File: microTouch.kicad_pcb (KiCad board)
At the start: 2 copper layers, 26.7 x 41.9 mm, 9 parts, among them J1 SERVO, J2 PRINTER, U1 T1302

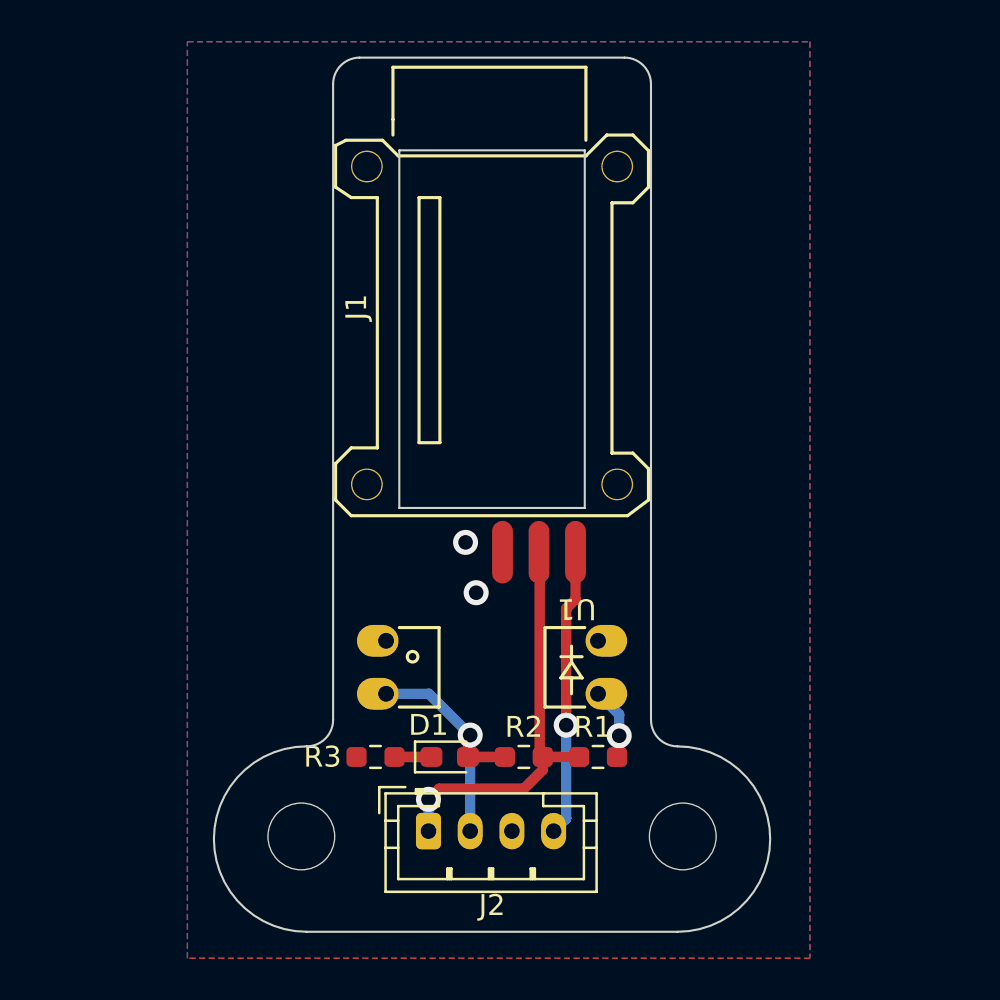
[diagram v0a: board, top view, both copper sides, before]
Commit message: smaller
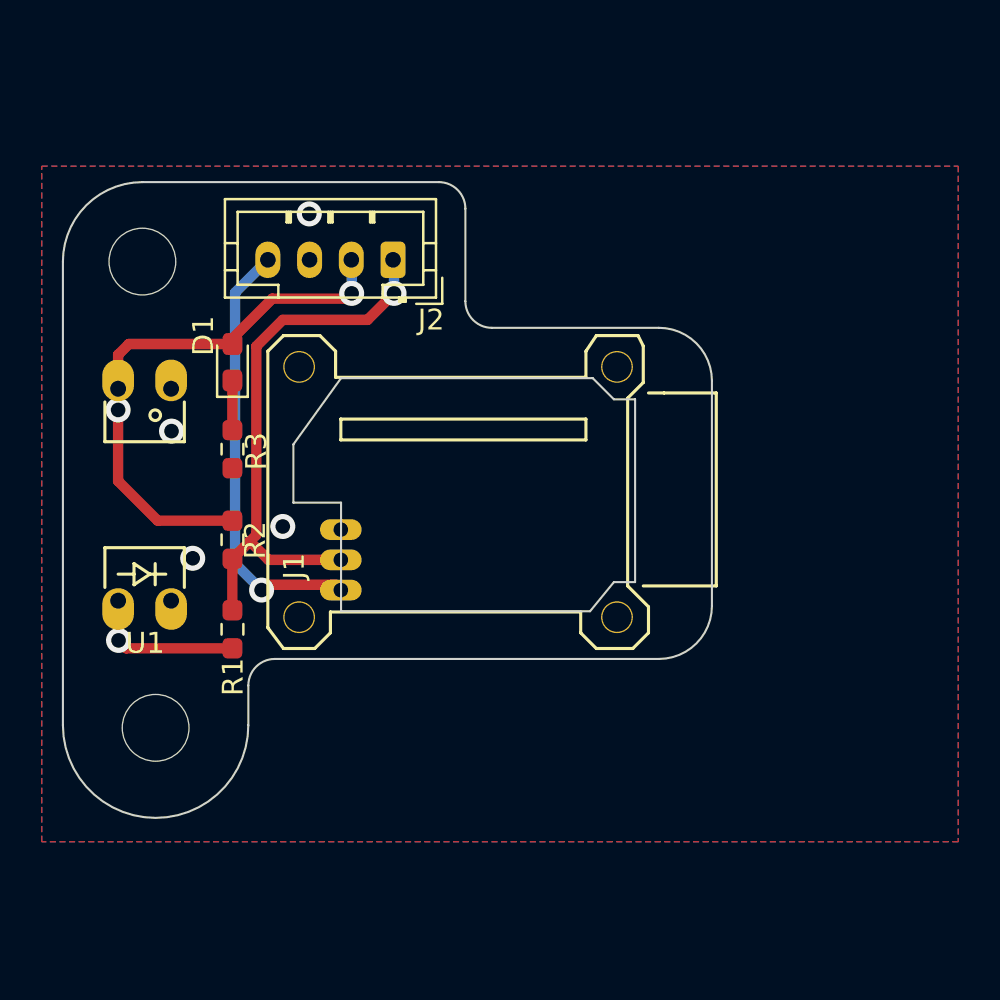
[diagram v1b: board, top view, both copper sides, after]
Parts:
- moved H1 28.6 mm to (102.2, 90.2), turned to 0 degrees
- moved J2 27.4 mm to (114.3, 90.1), turned to 180 degrees
- moved H2 25.8 mm to (102.9, 112.5), turned to 0 degrees
- moved D1 21.6 mm to (106.6, 95.0), turned to 90 degrees
- moved U1 20.6 mm to (103.6, 106.4), turned to 90 degrees
- moved R1 18.6 mm to (106.6, 107.8), turned to -90 degrees
- moved R2 17.4 mm to (106.6, 103.5), turned to -90 degrees
- moved R3 16.3 mm to (106.6, 99.2), turned to -90 degrees
- moved J1 6.50 mm to (109.7, 95.2), turned to 0 degrees
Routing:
- net /SIG: track 12.3 -> 26.5 mm, vias 1 -> 2
- net /VCC: track 19.8 -> 27.1 mm
- net /SERVO: track 13.8 -> 21.0 mm
- net Net-(R1-Pad2): track 3.50 -> 7.53 mm
- net Net-(D1-Pad1): track 1.77 -> 2.38 mm
- net GND: vias 2 -> 4
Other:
- board size 26.7 x 41.9 mm -> 31.1 x 30.5 mm
- board text added: "cperiod 2021"
- board text added: "microTouch v1.0"
- board text removed: "microTouch cperiod 2021"

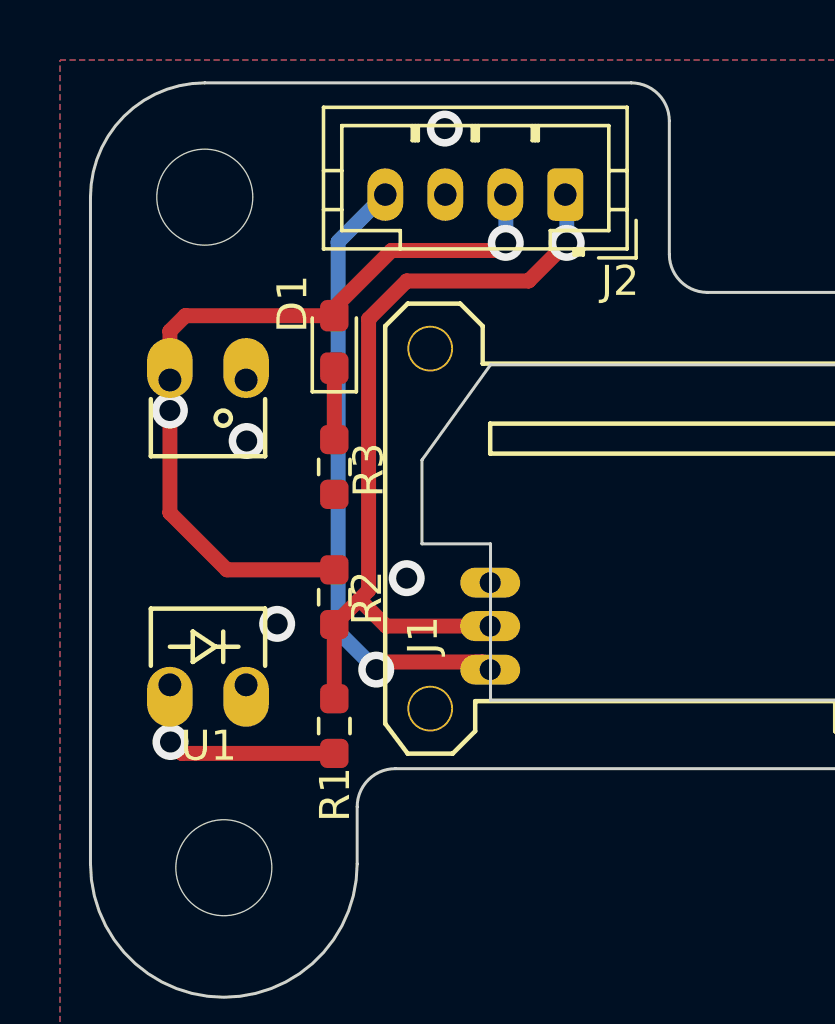
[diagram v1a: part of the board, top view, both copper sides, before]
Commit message: assorted tweaks
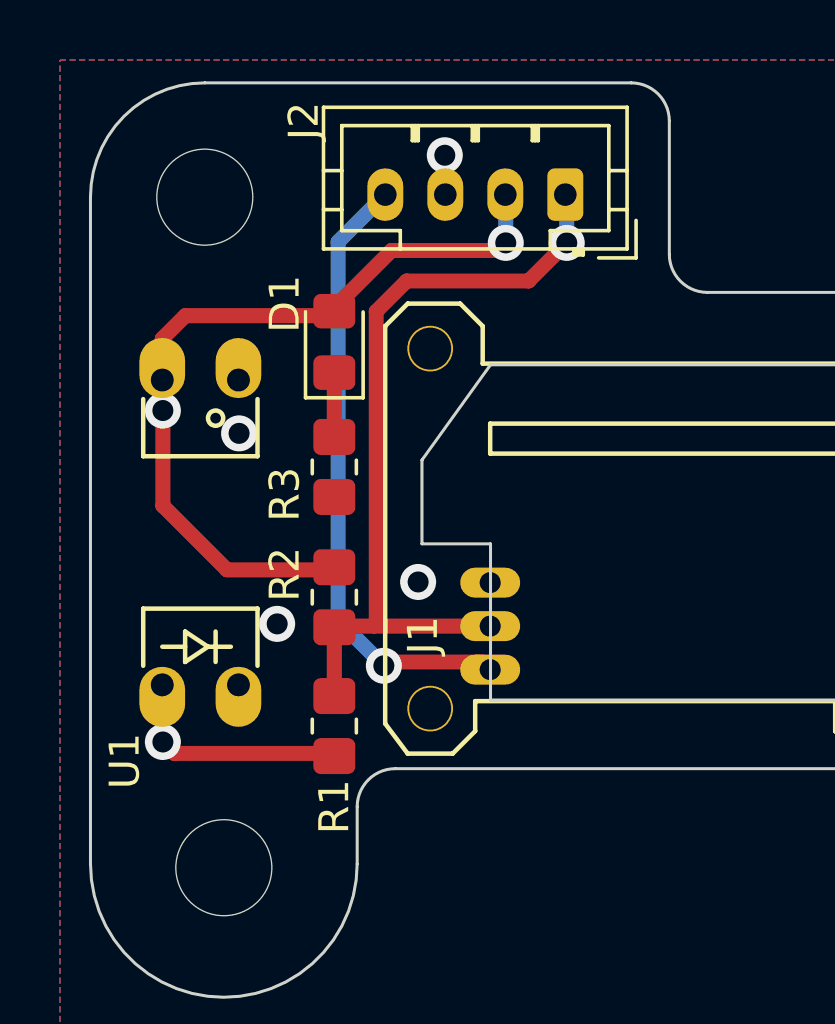
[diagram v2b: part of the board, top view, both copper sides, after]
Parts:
- D1: footprint LED_SMD:LED_0603_1608Metric_Pad1.05x0.95mm_HandSolder -> LED_SMD:LED_0805_2012Metric_Pad1.15x1.40mm_HandSolder
- R1, R2, R3: footprint Resistor_SMD:R_0603_1608Metric_Pad0.98x0.95mm_HandSolder -> Resistor_SMD:R_0805_2012Metric_Pad1.20x1.40mm_HandSolder
- moved U1 0.25 mm to (103.4, 106.4)
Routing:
- net Net-(R1-Pad2): track 7.53 -> 8.04 mm
